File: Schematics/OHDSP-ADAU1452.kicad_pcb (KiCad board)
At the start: 4 copper layers, 100 x 100 mm, 294 parts, among them CN201 COAX, CN401 COAX, CN402 COAX, CN405 COAX, CN406 COAX, P201 CONN_2x1, P203 CONN_6X2, P204 CONN_6x1, P301 CONN_2x1, P302 CONN_2x1, P303 PIN, P304 PIN, P305 PIN, P306 PIN, P601 CONN_02X05, P602 CONN_02X05, P603 CONN_02X05, P604 CONN_02X05, P605 CONN_3x1, P606 CONN_6X2, P607 CONN_02X05, P608 CONN_02X05, P609 CONN_02X20, P610 CONN_02X05, P611 CONN_5x1, P613 CONN_02X05, P614 CONN_02X05, P615 CONN_02X05, P616 CONN_02X05, SW202 SWITCH, U201 ADAU1452WBCPZ, U202 ADM13307-5ARZ, U203 25AA1024, U301 IC-REG-XRP7659ISTR-F, U302 IC-REG-XRP7659ISTR-F, U304 IC-REG-XC6210B332MR, U305 IC-REG-XC6210B332MR, U401 NB3L553, U501 IC-SPDIF-RX-OPTO, U502 IC-SPDIF-TX-OPTO, X201 24M576

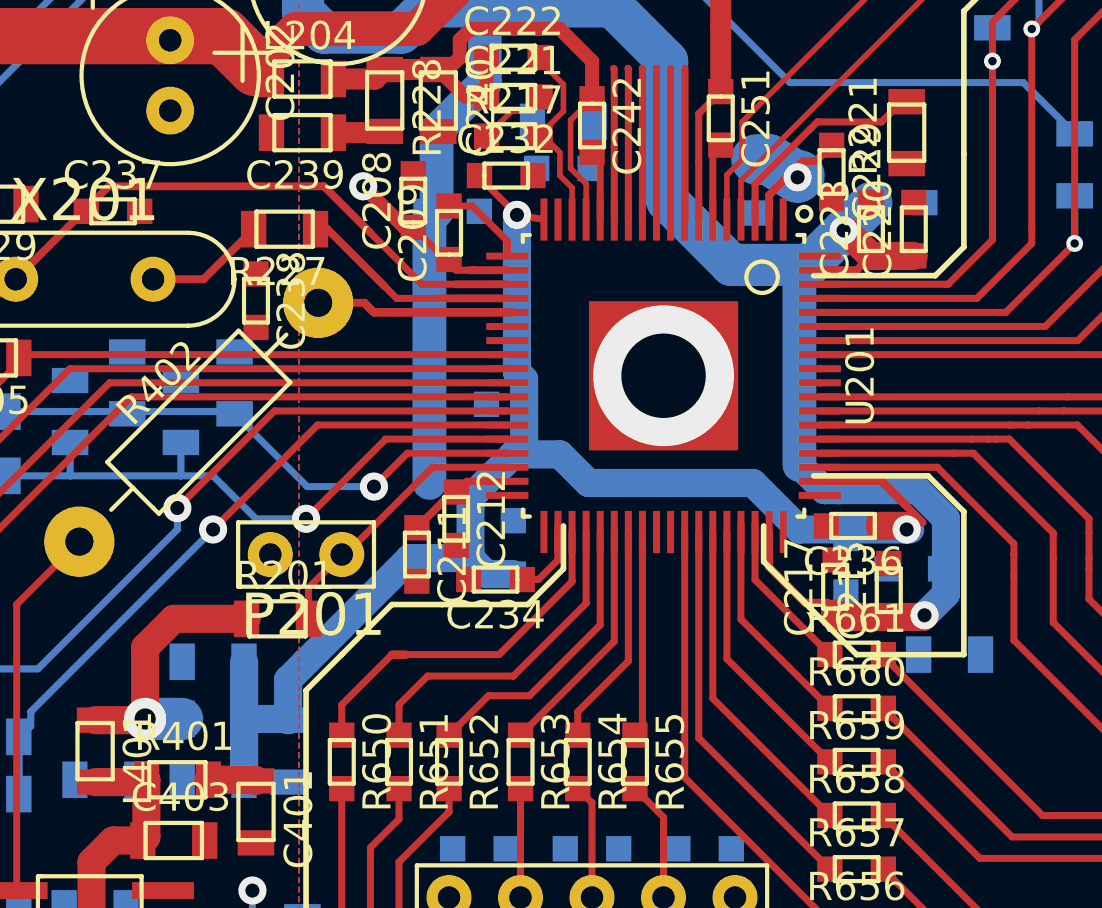
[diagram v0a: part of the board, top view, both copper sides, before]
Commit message: PCB work
Also playing with via sizes...
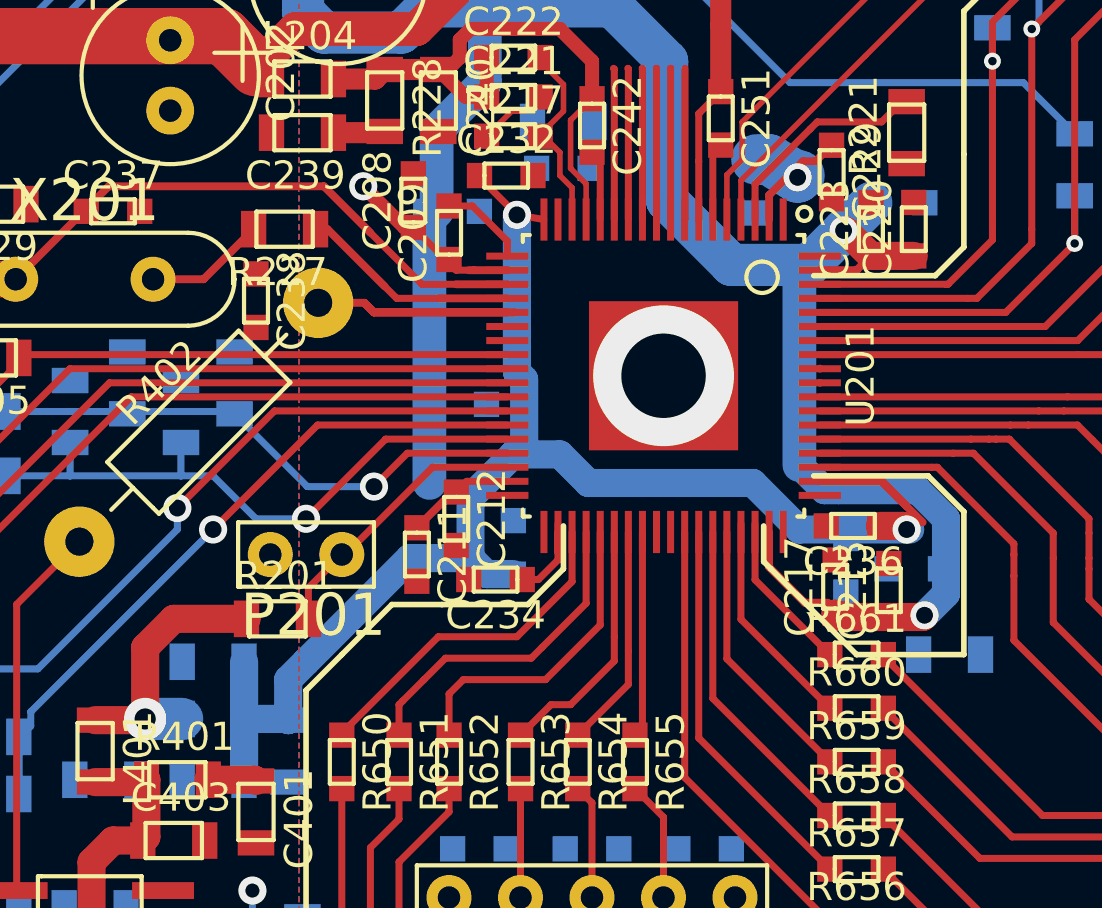
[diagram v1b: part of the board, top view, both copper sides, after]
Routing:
- net /ADAU1452/DACOUT_LRCLK0: track 13.9 -> 12.2 mm
- net /ADAU1452/DACOUT_SDATA0: track 10.3 -> 11.2 mm
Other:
- rule via_min_size: 0.6 -> 0.5
